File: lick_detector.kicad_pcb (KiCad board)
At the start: 2 copper layers, 19.3 x 19.3 mm, 16 parts, among them P1 CONN_FFC_8_VERT, P2 RECEPTACLE_2MM, U1 ADXL313, U2 BUFFER_TRI_STATE, U3 BUFFER_2_ELEMENT

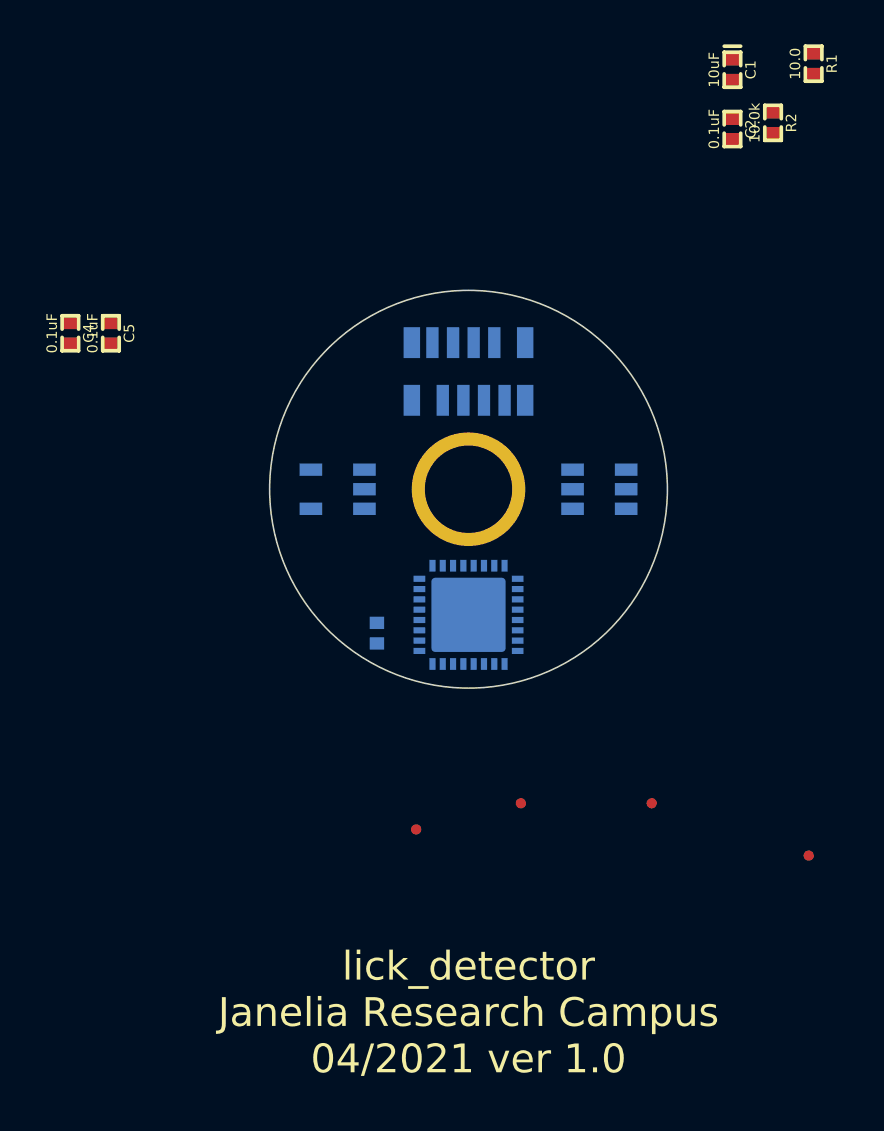
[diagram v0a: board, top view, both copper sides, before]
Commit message: Migrate toward 0201
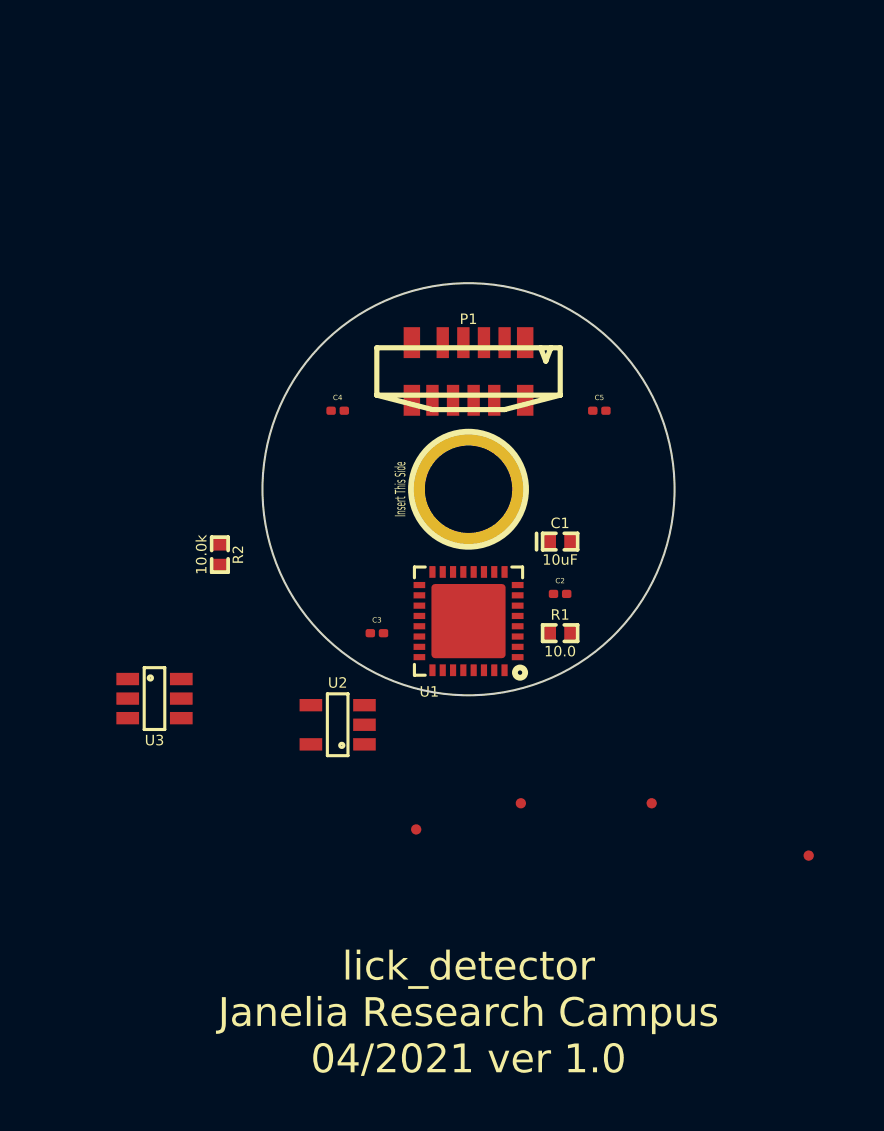
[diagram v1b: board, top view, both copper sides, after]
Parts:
- C2, C4, C5: footprint lick_detector:SM0402 -> lick_detector:C_0201_0603Metric
- C3: footprint lick_detector:SM0402 -> lick_detector:C_0201_0603Metric; moved to F.Cu
- P1, P2, U1, U2, U3: moved to F.Cu
- moved R2 34.1 mm to (114.9, 104.8)
- moved R1 30.3 mm to (131.4, 108.6), turned to 90 degrees
- moved C1 24.4 mm to (131.4, 104.1), turned to 90 degrees
- moved C2 24.1 mm to (131.4, 106.7)
- moved C5 24.0 mm to (133.3, 97.8)
- moved U3 23.9 mm to (111.8, 111.8), turned to 0 degrees
- moved C4 13.5 mm to (120.7, 97.8)
- moved U2 11.4 mm to (120.7, 113.0)
- moved U1 0.30 mm to (127.0, 108.0), turned to 180 degrees
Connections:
- U3 pad 2: (no net) -> GND
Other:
- board size 19.3 x 19.3 mm -> 20 x 20 mm
- net class Default: clearance 0.1016 -> 0.0762
- rule trace_clearance: 0.1016 -> 0.0762
